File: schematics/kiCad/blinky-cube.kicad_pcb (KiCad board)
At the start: 2 copper layers, 59 x 53 mm, 14 parts, among them J1 Screw_Terminal_01x02, J2 Screw_Terminal_01x03, J3 Screw_Terminal_01x03, SW1 SW_Push, U1 Pico

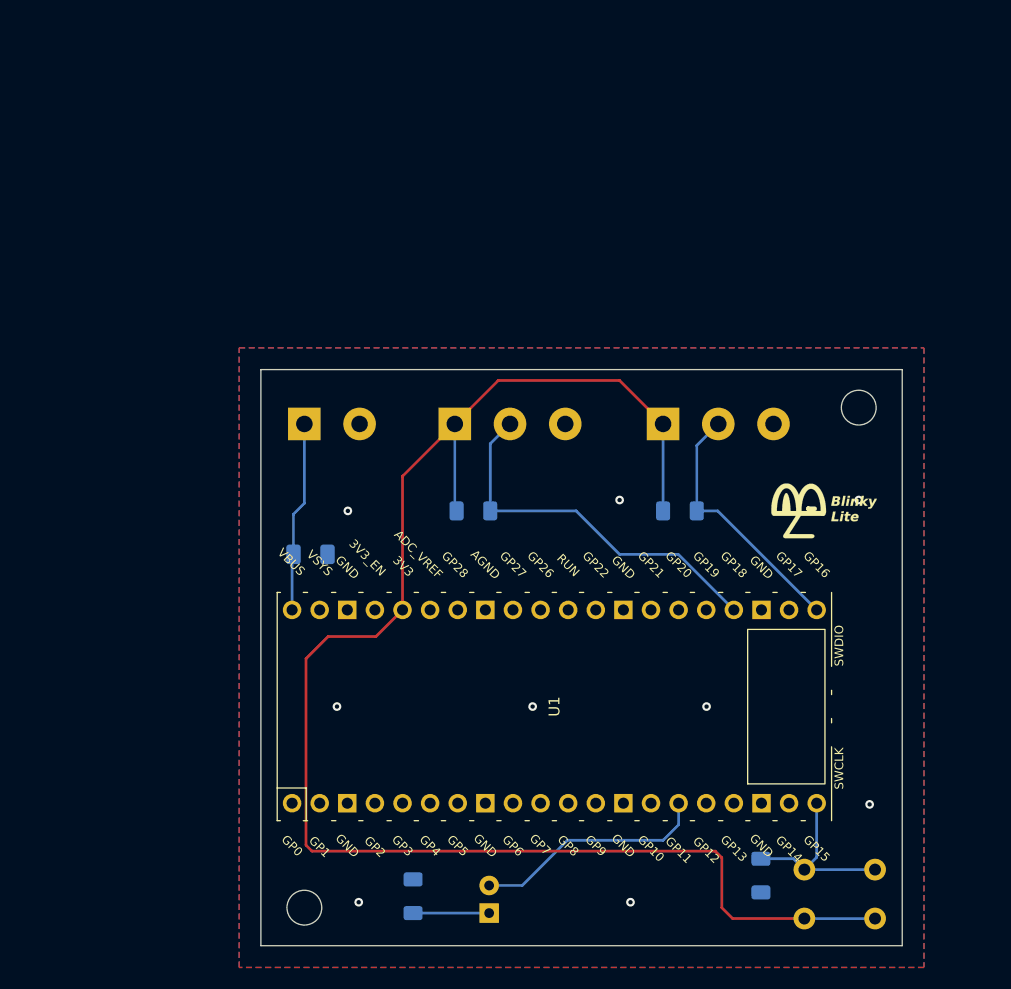
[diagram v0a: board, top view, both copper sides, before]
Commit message: schematic in DIN mode 3 format
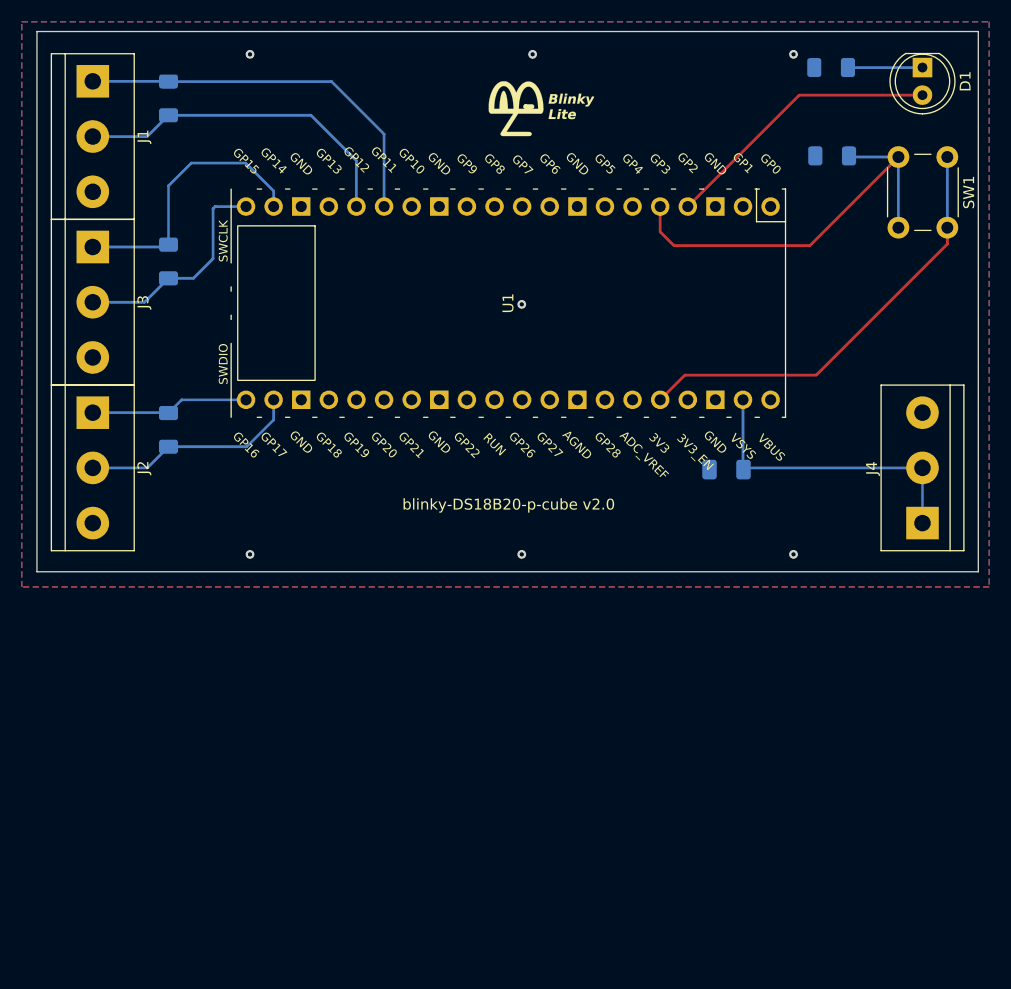
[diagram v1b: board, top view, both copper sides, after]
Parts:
- removed ? (x2): , 
- added J4: Screw_Terminal_01x03, TerminalBlock:TerminalBlock_bornier-3_P5.08mm, F.Cu at (181.9, 95.1)
- added R5: 10k, Resistor_SMD:R_1206_3216Metric_Pad1.30x1.75mm_HandSolder, B.Cu at (112.5, 86.5)
- D1, J2, J3, SW1: moved to F.Cu
- J1: value Screw_Terminal_01x02 -> Screw_Terminal_01x03; footprint TerminalBlock:TerminalBlock_bornier-2_P5.08mm -> TerminalBlock:TerminalBlock_bornier-3_P5.08mm; moved to F.Cu
- moved D1 87.4 mm to (181.9, 53.2), turned to -90 degrees
- moved R1 85.4 mm to (173.5, 53.2), turned to 0 degrees
- moved SW1 71.3 mm to (184.2, 61.4), turned to -90 degrees
- moved R2 66.5 mm to (173.6, 61.3), turned to 180 degrees
- moved J3 54.9 mm to (105.5, 69.7), turned to -90 degrees
- moved R4 52.3 mm to (112.5, 71.0), turned to 90 degrees
- moved R3 47.2 mm to (112.5, 56.0), turned to 90 degrees
- moved G*** 45.2 mm to (147.0, 57.0)
- moved C1 39.1 mm to (163.8, 90.2), turned to 180 degrees
- moved U1 37.4 mm to (143.8, 74.9), turned to -90 degrees
- moved J1 37.0 mm to (105.5, 54.5), turned to -90 degrees
- moved J2 33.3 mm to (105.5, 85.0), turned to -90 degrees
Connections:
- C1 pad 1: Net-(C1-Pad1) -> Net-(J4-Pin_1)
- D1 pad 2: Net-(D1-Pad2) -> Net-(D1-A)
- J1 pad 1: Net-(C1-Pad1) -> Net-(J1-Pin_1)
- J1 pad 2: GND -> Net-(J1-Pin_2)
- J2 pad 1: Net-(SW1-Pad1) -> Net-(J2-Pin_1)
- J2 pad 2: Net-(U1-Pad24) -> Net-(J2-Pin_2)
- J3 pad 1: Net-(SW1-Pad1) -> Net-(J3-Pin_1)
- J3 pad 2: Net-(U1-Pad21) -> Net-(J3-Pin_2)
- R2 pad 1: Net-(R2-Pad1) -> Net-(U1-GPIO3)
- R3 pad 1: Net-(U1-Pad24) -> Net-(J1-Pin_2)
- R3 pad 2: Net-(SW1-Pad1) -> Net-(J1-Pin_1)
- R4 pad 1: Net-(U1-Pad21) -> Net-(J3-Pin_2)
- R4 pad 2: Net-(SW1-Pad1) -> Net-(J3-Pin_1)
- SW1 pad 1: Net-(SW1-Pad1) -> Net-(U1-3V3)
- SW1 pad 2: Net-(R2-Pad1) -> Net-(U1-GPIO3)
- U1 pad 15: Net-(D1-Pad2) -> Net-(J1-Pin_1)
- U1 pad 16: unconnected-(U1-Pad16) -> Net-(J1-Pin_2)
- U1 pad 19: unconnected-(U1-Pad19) -> Net-(J3-Pin_1)
- U1 pad 20: Net-(R2-Pad1) -> Net-(J3-Pin_2)
- U1 pad 21: Net-(U1-Pad21) -> Net-(J2-Pin_1)
- U1 pad 22: unconnected-(U1-Pad22) -> Net-(J2-Pin_2)
- U1 pad 24: Net-(U1-Pad24) -> unconnected-(U1-GPIO18-Pad24)
- U1 pad 36: Net-(SW1-Pad1) -> Net-(U1-3V3)
- U1 pad 39: unconnected-(U1-Pad39) -> Net-(J4-Pin_1)
- U1 pad 4: unconnected-(U1-Pad4) -> Net-(D1-A)
- U1 pad 40: Net-(C1-Pad1) -> unconnected-(U1-VBUS-Pad40)
- U1 pad 5: unconnected-(U1-Pad5) -> Net-(U1-GPIO3)
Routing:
- net Net-(SW1-Pad1): track 143.4 -> 0.00 mm
- net Net-(U1-3V3): track 0.00 -> 40.4 mm
- net Net-(U1-GPIO3): track 0.00 -> 39.2 mm
- net Net-(J1-Pin_1): track 0.00 -> 35.5 mm
- net Net-(U1-Pad24): track 34.9 -> 0.00 mm
- net Net-(J1-Pin_2): track 0.00 -> 31.0 mm
- net Net-(J4-Pin_1): track 0.00 -> 28.0 mm
- net Net-(D1-A): track 0.00 -> 25.8 mm
- net Net-(J3-Pin_1): track 0.00 -> 25.5 mm
- net Net-(U1-Pad21): track 23.6 -> 0.00 mm
- net Net-(D1-Pad2): track 21.7 -> 0.00 mm
- net Net-(J3-Pin_2): track 0.00 -> 20.4 mm
- net Net-(J2-Pin_2): track 0.00 -> 20.3 mm
- net Net-(C1-Pad1): track 17.7 -> 0.00 mm
- net Net-(R2-Pad1): track 17.5 -> 0.00 mm
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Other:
- board size 59 x 53 mm -> 86.6 x 49.7 mm
- board text added: "blinky-DS18B20-p-cube v2.0"
